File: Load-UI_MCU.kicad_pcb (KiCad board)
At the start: 4 copper layers, 85 x 90 mm, 116 parts, among them IC1 MSPM0G3519SPMR, IC2 TPS73533DRVT, IC3 TC4429CPA, IC4 TPS2121RUXR, J1 Conn_01x05_Socket, J10 Conn_01x02_Socket, J11 Conn_01x02_Socket, J12 Conn_01x02_Socket, J13 Conn_01x02_Socket, J14 Conn_01x02_Socket, J15 Conn_01x08_Pin, J16 Conn_01x02_Socket, J19 Conn_01x03_Socket, J2 Conn_01x06_Socket, J20 Conn_01x02_Socket, J21 Conn_01x02_Socket, J22 Conn_01x02_Socket, J23 Conn_01x02_Socket, J24 Conn_01x02_Socket, J3 Conn_01x02_Socket, J4 Conn_01x06_Socket, J5 Conn_01x02_Socket, J6 Conn_01x02_Socket, J7 Conn_01x02_Socket, J8 Conn_01x06_Socket, J9 Conn_01x03_Socket, Q2 2N2219, SW1 SW_Push, SW2 SW_Push, SW3 SW_Push_DPDT, U1 INA229AQDGSRQ1, U2 INA229AQDGSRQ1, U3 SN74HC14N, U4 SN74HC14N

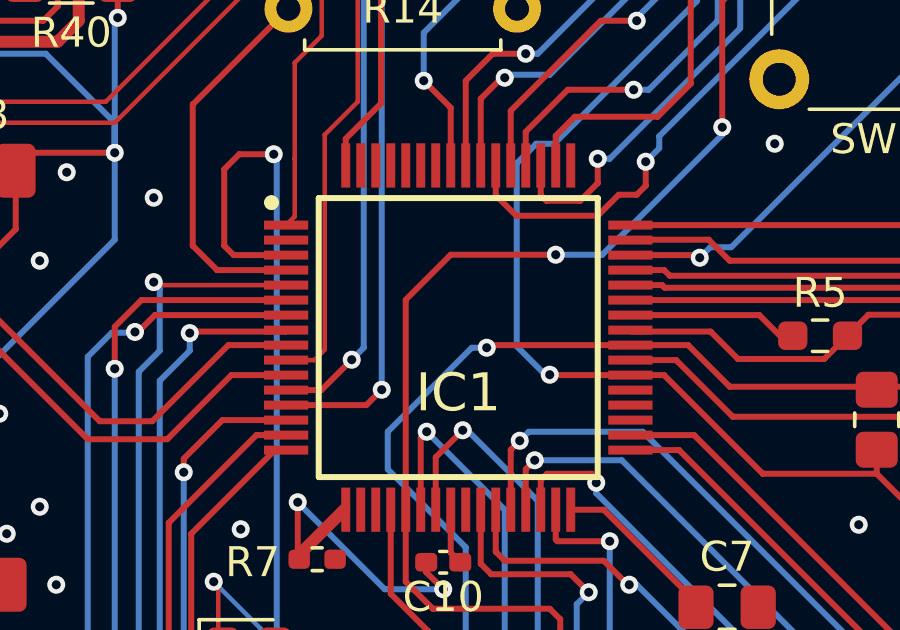
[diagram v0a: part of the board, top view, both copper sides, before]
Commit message: EE
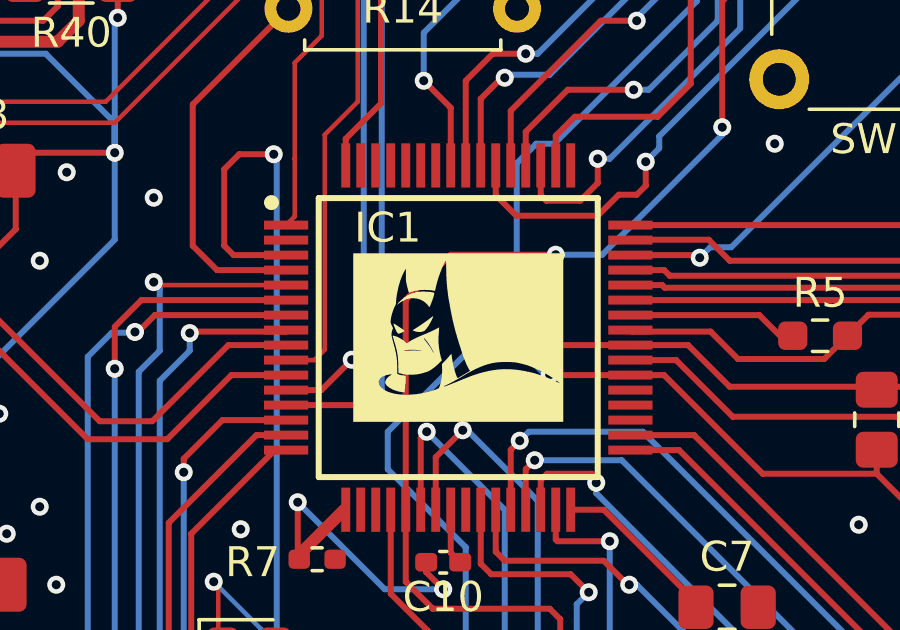
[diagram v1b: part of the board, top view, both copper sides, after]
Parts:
- added G***: LOGO, LOGO, F.Cu at (154.7, 84.8)
